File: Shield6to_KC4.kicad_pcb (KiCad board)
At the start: 2 copper layers, 90 x 62 mm, 22 parts, among them J1 DB9, P1 CONN_9, P2 CONN_8, P3 CONN_9, P4 CONN_8, P5 CONN_8, P6 CONN_8, P7 CONN_8, P8 CONN_8, U1 ID-12LA, U2 MAX232

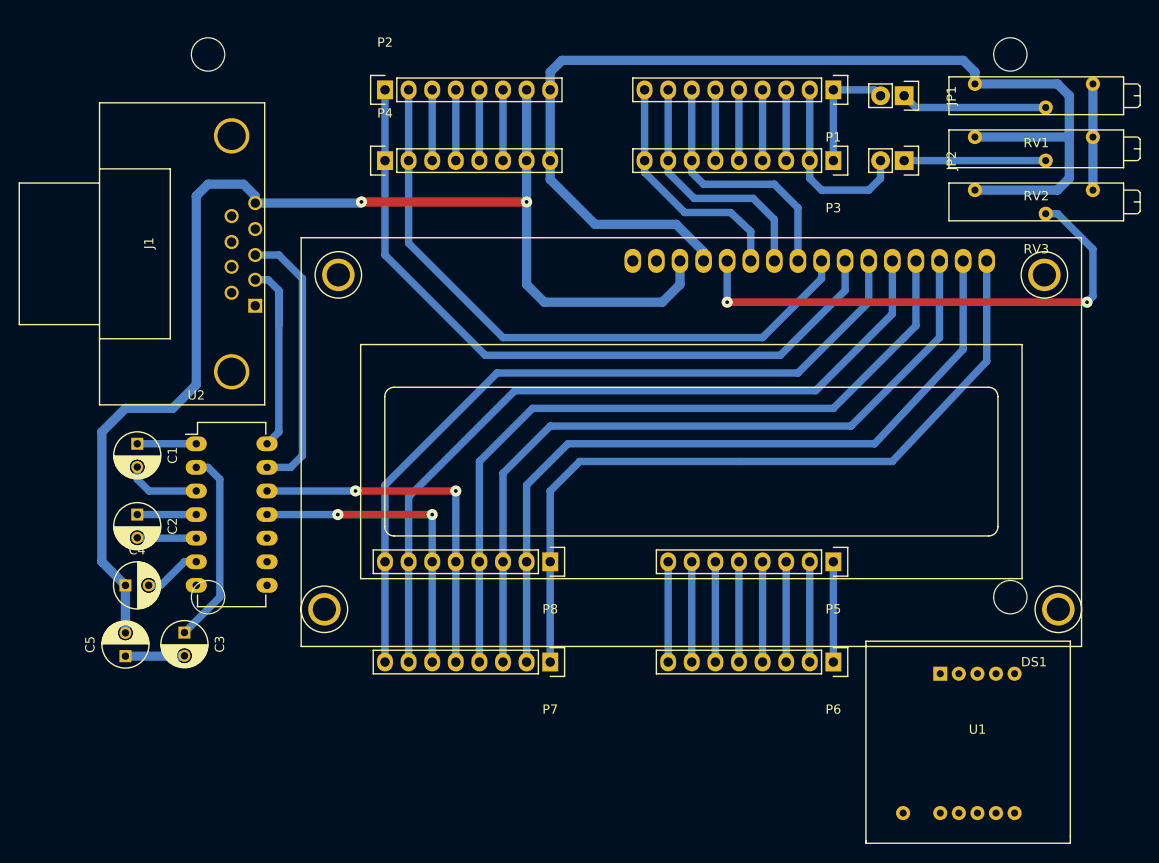
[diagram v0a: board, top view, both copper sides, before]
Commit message: Primera version de la Placa lista para la Revision de MArtín
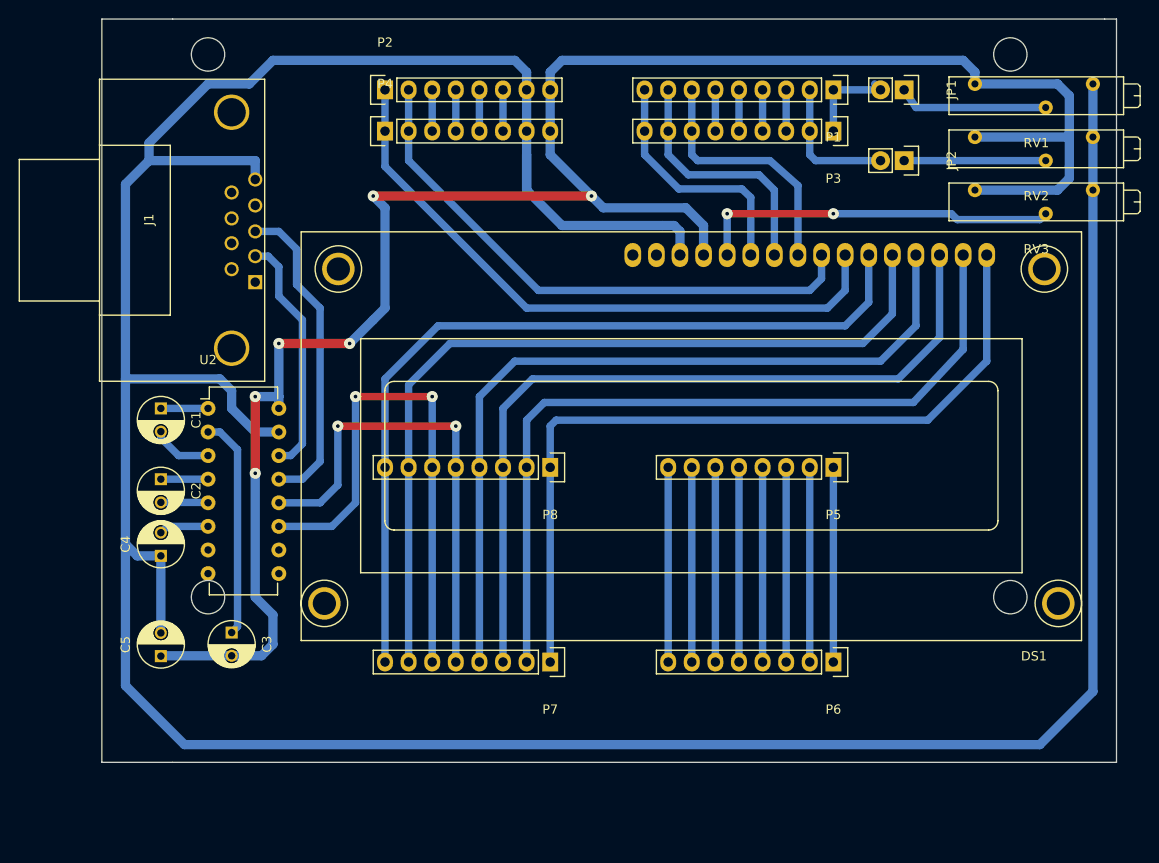
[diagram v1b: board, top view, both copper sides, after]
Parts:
- removed U1: ID-12LA, Librerias:ID12-LA
- U2: footprint Housings_DIP:DIP-14_W7.62mm_LongPads -> Housings_DIP:DIP-16_W7.62mm
- moved P5 10.2 mm to (137.2, 101.6)
- moved P8 10.2 mm to (106.7, 101.6)
- moved C3 5.08 mm to (72.4, 119.4)
- moved C4 4.96 mm to (64.8, 111.1), turned to 90 degrees
- moved C1 4.58 mm to (64.8, 95.2)
- moved C2 4.58 mm to (64.8, 102.9)
- moved U2 4.02 mm to (69.8, 95.2)
- moved C5 3.81 mm to (64.8, 121.9)
- moved P3 3.17 mm to (137.2, 65.4)
- moved P4 3.17 mm to (88.9, 65.4)
- moved J1 2.54 mm to (73.7, 76.2)
- moved DS1 0.64 mm to (120.7, 78.7)
- moved JP1 0.63 mm to (144.8, 61.0)
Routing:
- net GND: track 146.3 -> 363.0 mm, vias 2 -> 0
- net +5V: track 127.1 -> 218.9 mm, vias 0 -> 6
- net TX: track 33.7 -> 57.6 mm
- net Net-(DS1-Pad3): track 55.8 -> 39.3 mm
- net RX: track 39.4 -> 52.2 mm
- net /RB7: track 10.8 -> 21.0 mm
- net /RB6: track 10.8 -> 21.0 mm
- net /RB5: track 10.8 -> 21.0 mm
- net /RB4: track 10.8 -> 21.0 mm
- net /RB3: track 10.8 -> 21.0 mm
- net /RB2: track 10.8 -> 21.0 mm
- net /RB1: track 10.8 -> 21.0 mm
- net /RB0: track 10.8 -> 21.0 mm
- net /RD1: track 77.8 -> 68.7 mm
- net /RD0: track 69.7 -> 60.9 mm
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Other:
- board size 90 x 62 mm -> 109.2 x 80 mm
